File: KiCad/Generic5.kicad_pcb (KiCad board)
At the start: 2 copper layers, 12.5 x 31 mm, 26 parts, among them J1 Conn_01x04, J2 USB-C, U1 ESP32-PICO-MINI-02, U2 FT231XQ, U3 LMR16006+FB

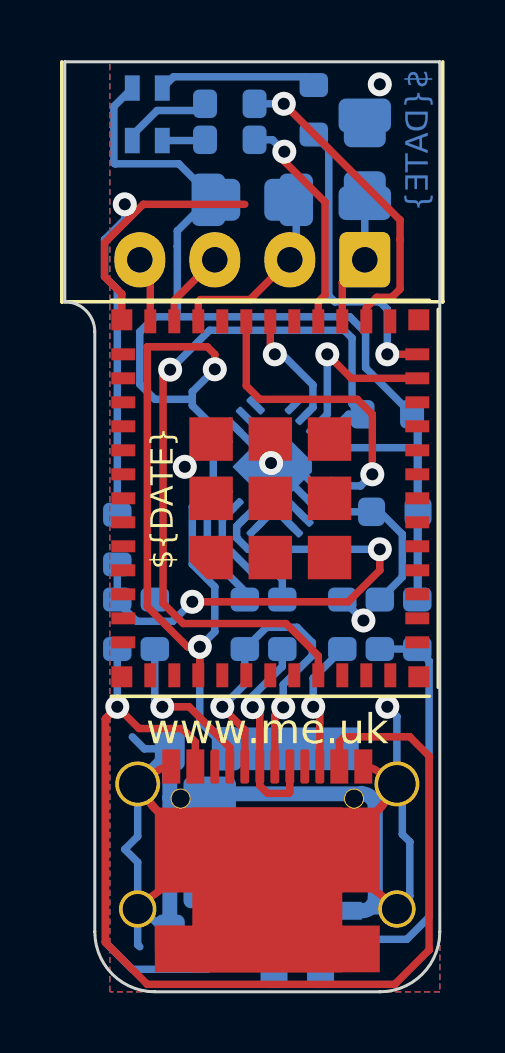
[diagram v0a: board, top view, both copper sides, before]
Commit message: Tidy tracks
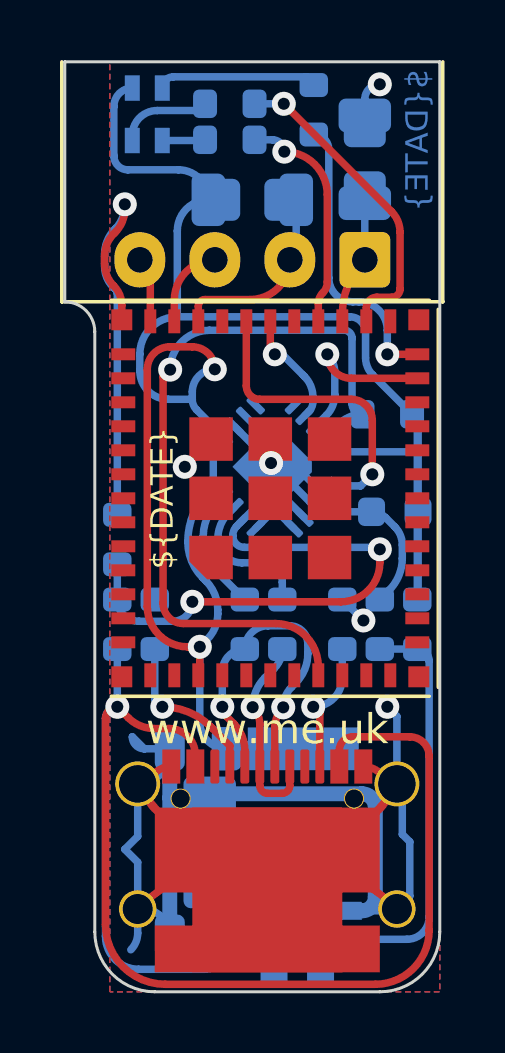
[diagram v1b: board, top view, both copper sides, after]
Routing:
- net GND: track 57.4 -> 55.6 mm
- net +3V3: track 70.4 -> 69.7 mm
